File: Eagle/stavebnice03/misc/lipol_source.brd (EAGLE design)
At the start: 25 parts

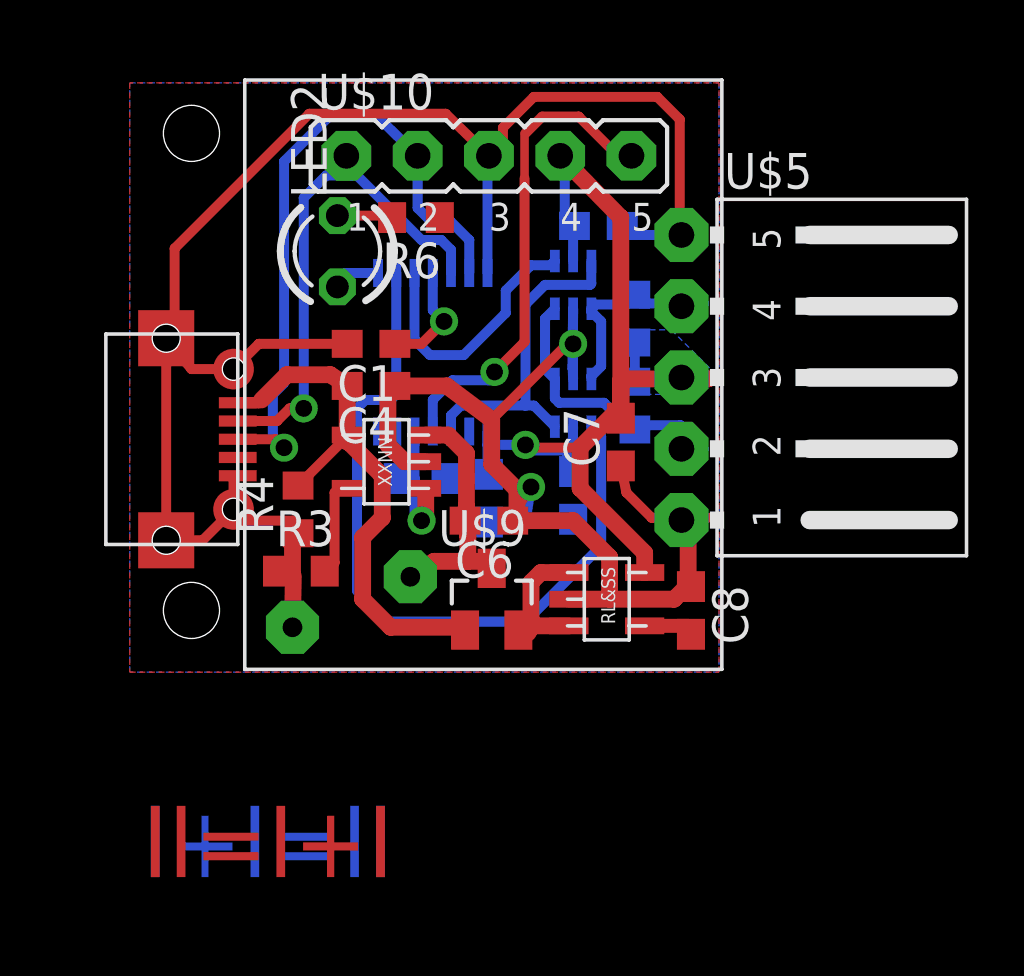
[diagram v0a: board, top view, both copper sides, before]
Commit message: minor element position changes
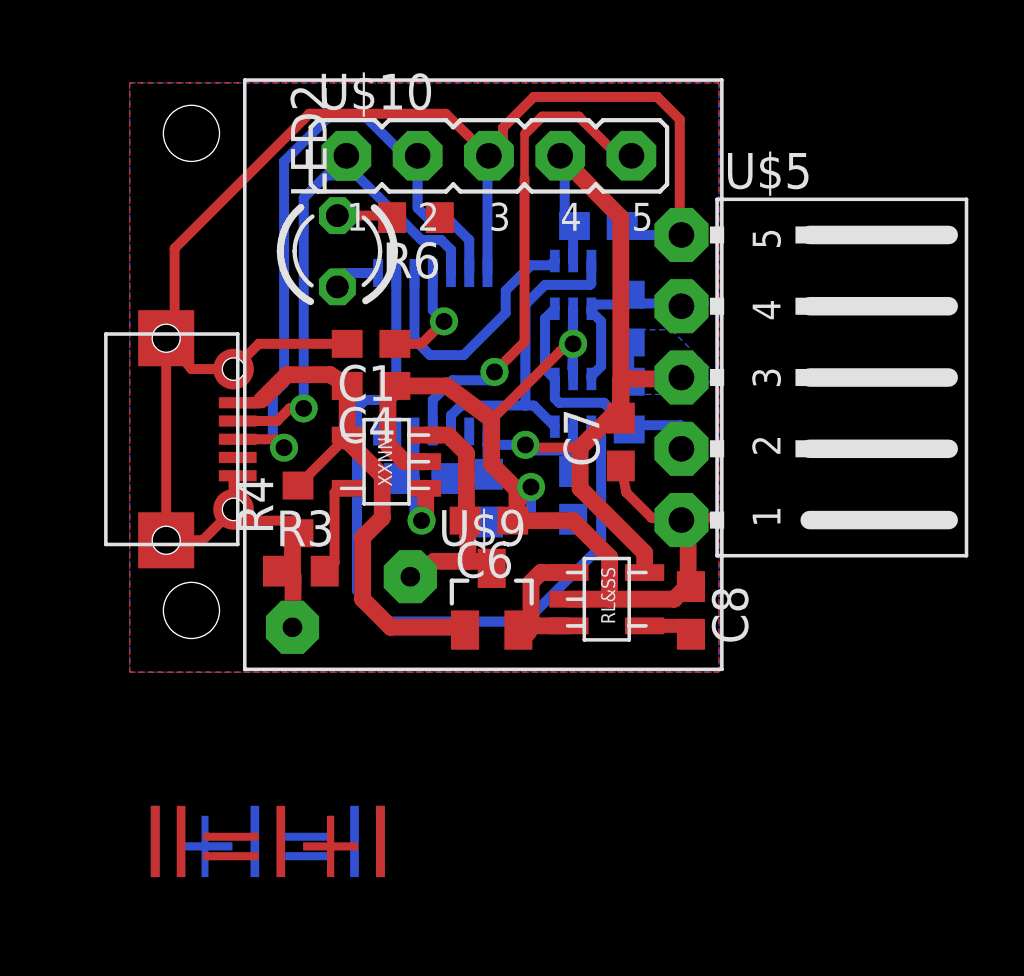
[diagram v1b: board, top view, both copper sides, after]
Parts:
- moved R1 0.20 mm to (17.8, 9.50)
- moved R2 0.20 mm to (17.8, 12.6)
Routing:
- net VCC: track 42.8 -> 39.6 mm
- net N$6: track 10.5 -> 9.58 mm
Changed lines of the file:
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@@
 <layers>
 <layer number="1" name="Top" color="4" fill="1" visible="yes" active="yes"/>
-<layer number="16" name="Bottom" color="1" fill="1" visible="yes" active="yes"/>
+<layer number="16" name="Bottom" color="1" fill="1" visible="no" active="yes"/>
 <layer number="17" name="Pads" color="2" fill="1" visible="yes" active="yes"/>
 <layer number="18" name="Vias" color="2" fill="1" visible="yes" active="yes"/>
 <layer number="19" name="Unrouted" color="6" fill="1" visible="yes" active="yes"/>
 <layer number="20" name="Dimension" color="15" fill="1" visible="yes" active="yes"/>
-<layer number="21" name="tPlace" color="7" fill="1" visible="yes" active="yes"/>
-<layer number="22" name="bPlace" color="7" fill="1" visible="yes" active="yes"/>
+<layer number="21" name="tPlace" color="7" fill="1" visible="no" active="yes"/>
+<layer number="22" name="bPlace" color="7" fill="1" visible="no" active="yes"/>
 <layer number="23" name="tOrigins" color="15" fill="1" visible="yes" active="yes"/>
 <layer number="24" name="bOrigins" color="15" fill="1" visible="yes" active="yes"/>
@@
 <layer number="43" name="vRestrict" color="2" fill="10" visible="no" active="yes"/>
 <layer number="44" name="Drills" color="7" fill="1" visible="no" active="yes"/>
-<layer number="45" name="Holes" color="7" fill="1" visible="yes" active="yes"/>
+<layer number="45" name="Holes" color="7" fill="1" visible="no" active="yes"/>
 <layer number="46" name="Milling" color="3" fill="1" visible="no" active="yes"/>
 <layer number="47" name="Measures" color="7" fill="1" visible="no" active="yes"/>
@@
 <vertex x="13" y="2.8"/>
 </polygon>
-<wire x1="-2" y1="-2.5" x2="24" y2="-2.5" width="0.01" layer="49"/>
-<wire x1="24" y1="-2.5" x2="24" y2="23.5" width="0.01" layer="49"/>
-<wire x1="24" y1="23.5" x2="-2" y2="23.5" width="0.01" layer="49"/>
-<wire x1="-2" y1="23.5" x2="-2" y2="-2.5" width="0.01" layer="49"/>
-<text x="5.1" y="27.3" size="1.778" layer="49">Lipol source</text>
+<wire x1="-10" y1="-10" x2="31" y2="-10" width="0.01" layer="49"/>
+<wire x1="31" y1="-10" x2="31" y2="31" width="0.01" layer="49"/>
+<wire x1="31" y1="31" x2="-10" y2="31" width="0.01" layer="49"/>
+<wire x1="-10" y1="31" x2="-10" y2="-10" width="0.01" layer="49"/>
+<text x="10.5" y="27" size="1.778" layer="49" align="center">Lipol source</text>
 <circle x="2.2" y="19.2" radius="0.6" width="0.9" layer="116"/>
 <circle x="2.2" y="2.2" radius="0.6" width="0.9" layer="116"/>
@@
 <element name="U$1" library="!stavebnice03" package="TSSOP14" value="16F1454" x="10.8" y="11.4" rot="MR0"/>
 <element name="C2" library="resistor" package="C0603" value="100nF" x="12.8" y="6.2" rot="MR270"/>
-<element name="R1" library="resistor" package="R0603" value="2k2" x="18" y="9.5" rot="MR90"/>
-<element name="R2" library="resistor" package="R0603" value="2k2" x="18" y="12.6" rot="MR270"/>
+<element name="R1" library="resistor" package="R0603" value="2k2" x="17.8" y="9.5" rot="MR90"/>
+<element name="R2" library="resistor" package="R0603" value="2k2" x="17.8" y="12.6" rot="MR270"/>
 <element name="C3" library="resistor" package="C0603" value="100nF" x="16.7" y="15.9" rot="MR0"/>
 <element name="U$5" library="!stavebnice03" package="JUMPER5F-90" value="JUMPER5F-90" x="22.2" y="10.5" rot="R270"/>
@@
 <wire x1="7.75" y1="11.7" x2="4.6" y2="11.7" width="0.357" layer="1"/>
 <wire x1="4.6" y1="11.7" x2="3.7" y2="10.8" width="0.357" layer="1"/>
-<wire x1="12.8" y1="5.35" x2="14.1" y2="5.35" width="0.357" layer="16"/>
-<wire x1="14.1" y1="5.35" x2="15.8" y2="5.45" width="0.357" layer="16"/>
-<wire x1="15.8" y1="5.45" x2="15.3" y2="5.4" width="0.357" layer="16"/>
+<wire x1="12.8" y1="5.35" x2="14.3" y2="5.35" width="0.357" layer="16"/>
+<wire x1="14.3" y1="5.35" x2="15.8" y2="5.45" width="0.357" layer="16"/>
+<wire x1="15.8" y1="5.45" x2="15.8" y2="5.5" width="0.357" layer="16"/>
 <via x="14.3" y="6.6" extent="1-16" drill="0.6"/>
-<wire x1="14.1" y1="5.35" x2="14.3" y2="6.6" width="0.357" layer="16"/>
+<wire x1="14.3" y1="5.35" x2="14.3" y2="6.6" width="0.357" layer="16"/>
 <wire x1="13.8" y1="6.5" x2="13.8" y2="6.1" width="0.357" layer="1"/>
 <wire x1="13.8" y1="6.1" x2="13.9" y2="6" width="0.357" layer="1"/>
@@
 <wire x1="12.75" y1="7.2" x2="12.8" y2="7.05" width="0.3556" layer="16"/>
 <wire x1="14.1" y1="8.1" x2="12.75" y2="8.1" width="0.3556" layer="16"/>
-<wire x1="18" y1="10.35" x2="18" y2="11.75" width="0.3556" layer="16"/>
+<wire x1="17.8" y1="10.35" x2="17.8" y2="11.75" width="0.3556" layer="16"/>
 <contactref element="TC1185" pad="VOUT"/>
 <contactref element="C7" pad="2"/>
@@
 <wire x1="16.05" y1="8" x2="16.05" y2="6.55" width="0.6" layer="1"/>
 <wire x1="18.35" y1="4.25" x2="16.05" y2="6.55" width="0.6" layer="1"/>
-<wire x1="20.51" y1="10.35" x2="18" y2="10.35" width="0.3556" layer="16"/>
+<wire x1="19.51" y1="10.35" x2="17.8" y2="10.35" width="0.3556" layer="16"/>
 <wire x1="15.8" y1="14.65" x2="15.8" y2="15.85" width="0.3556" layer="16"/>
 <wire x1="15.8" y1="15.85" x2="15.85" y2="15.9" width="0.3556" layer="16"/>
@@
 <wire x1="12.55" y1="6.9" x2="12.8" y2="7.05" width="0.3556" layer="16"/>
 <wire x1="15.85" y1="15.9" x2="15.7" y2="15.9" width="0.3556" layer="16"/>
-<wire x1="20.51" y1="10.35" x2="19.66" y2="10.5" width="0.3556" layer="16"/>
+<wire x1="19.51" y1="10.35" x2="19.66" y2="10.5" width="0.3556" layer="16"/>
 <wire x1="17.19" y1="9.14" x2="16.05" y2="8" width="0.6" layer="1"/>
 <wire x1="17.5" y1="16.2" x2="17.5" y2="9.05" width="0.6" layer="1"/>
 <wire x1="17.5" y1="9.05" x2="17.51" y2="10.45" width="0.6" layer="1"/>
-<wire x1="17.51" y1="10.45" x2="20.61" y2="10.45" width="0.6" layer="1"/>
-<wire x1="20.61" y1="10.45" x2="19.66" y2="10.5" width="0.6" layer="1"/>
+<wire x1="17.51" y1="10.45" x2="19.71" y2="10.45" width="0.6" layer="1"/>
+<wire x1="19.71" y1="10.45" x2="19.66" y2="10.5" width="0.6" layer="1"/>
 <wire x1="17.19" y1="9.14" x2="17.69" y2="9.04" width="0.357" layer="1"/>
 <wire x1="17.69" y1="9.04" x2="17.5" y2="9.05" width="0.357" layer="1"/>
@@
 <wire x1="16.45" y1="12.95" x2="16.45" y2="12.85" width="0.3556" layer="16"/>
 <wire x1="16.45" y1="12.85" x2="16.8" y2="12.5" width="0.3556" layer="16"/>
-<wire x1="18.21" y1="13.14" x2="18" y2="13.45" width="0.3556" layer="16"/>
-<wire x1="18" y1="13.45" x2="17.9" y2="13.3" width="0.3556" layer="16"/>
+<wire x1="18.21" y1="13.14" x2="17.8" y2="13.45" width="0.3556" layer="16"/>
+<wire x1="17.8" y1="13.45" x2="17.9" y2="13.3" width="0.3556" layer="16"/>
 <wire x1="17.9" y1="13.3" x2="17.7" y2="13.1" width="0.3556" layer="16"/>
 <wire x1="18.21" y1="13.14" x2="20.46" y2="13.14" width="0.3556" layer="16"/>
@@
 <wire x1="14.8" y1="12.6" x2="14.8" y2="10.795" width="0.357" layer="16"/>
 <wire x1="14.8" y1="10.795" x2="15.15" y2="10.45" width="0.357" layer="16"/>
-<wire x1="18" y1="8.65" x2="18.1" y2="8.8" width="0.3556" layer="16"/>
+<wire x1="17.8" y1="8.65" x2="18.1" y2="8.8" width="0.3556" layer="16"/>
 <wire x1="18.1" y1="8.8" x2="19.62" y2="8.8" width="0.3556" layer="16"/>
-<wire x1="18" y1="8.65" x2="17.95" y2="8.75" width="0.3556" layer="16"/>
+<wire x1="17.8" y1="8.65" x2="17.95" y2="8.75" width="0.3556" layer="16"/>
 <wire x1="17.95" y1="8.75" x2="17.9" y2="8.8" width="0.3556" layer="16"/>
 <wire x1="17.9" y1="8.8" x2="17.7" y2="8.8" width="0.3556" layer="16"/>
@@
 <wire x1="15.15" y1="9.75" x2="15.3" y2="9.6" width="0.3556" layer="16"/>
 <wire x1="15.3" y1="9.6" x2="16.9" y2="9.6" width="0.3556" layer="16"/>
-<wire x1="20.46" y1="7.96" x2="19.66" y2="7.96" width="0.3556" layer="16"/>
-<wire x1="19.62" y1="8.8" x2="20.46" y2="7.96" width="0.3556" layer="16"/>
+<wire x1="19.66" y1="8.06" x2="19.66" y2="7.96" width="0.3556" layer="16"/>
+<wire x1="19.62" y1="8.8" x2="19.66" y2="8.06" width="0.3556" layer="16"/>
 </signal>
 <signal name="N$7">
@@
 <wire x1="10.7" y1="16.1" x2="10.26" y2="16.54" width="0.357" layer="16"/>
 <wire x1="10.26" y1="16.54" x2="10.26" y2="18.4" width="0.357" layer="16"/>
-<wire x1="8.82" y1="19.8" x2="10.26" y2="18.4" width="0.357" layer="16"/>
 <wire x1="5.5" y1="10.3" x2="5.5" y2="18.2" width="0.3556" layer="16"/>
 <wire x1="5.5" y1="18.2" x2="7.1" y2="19.8" width="0.3556" layer="16"/>
-<wire x1="7.1" y1="19.8" x2="8.82" y2="19.8" width="0.3556" layer="16"/>
+<wire x1="7.1" y1="19.8" x2="8.4" y2="19.8" width="0.3556" layer="16"/>
+<wire x1="8.4" y1="19.8" x2="9.7" y2="18.5" width="0.3556" layer="16"/>
+<wire x1="9.7" y1="18.5" x2="10.16" y2="18.5" width="0.3556" layer="16"/>
+<wire x1="10.16" y1="18.5" x2="10.26" y2="18.4" width="0.3556" layer="16"/>
 </signal>
 <signal name="N$3">
